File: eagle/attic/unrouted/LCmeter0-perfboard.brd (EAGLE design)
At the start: 51.1 x 49.5 mm, 25 parts, among them IC1 PIC16F876A-X/SP, K2 DS2Y, Q1 20MHz, Q2 BC548, SW1 SPST, SW2 DPDT

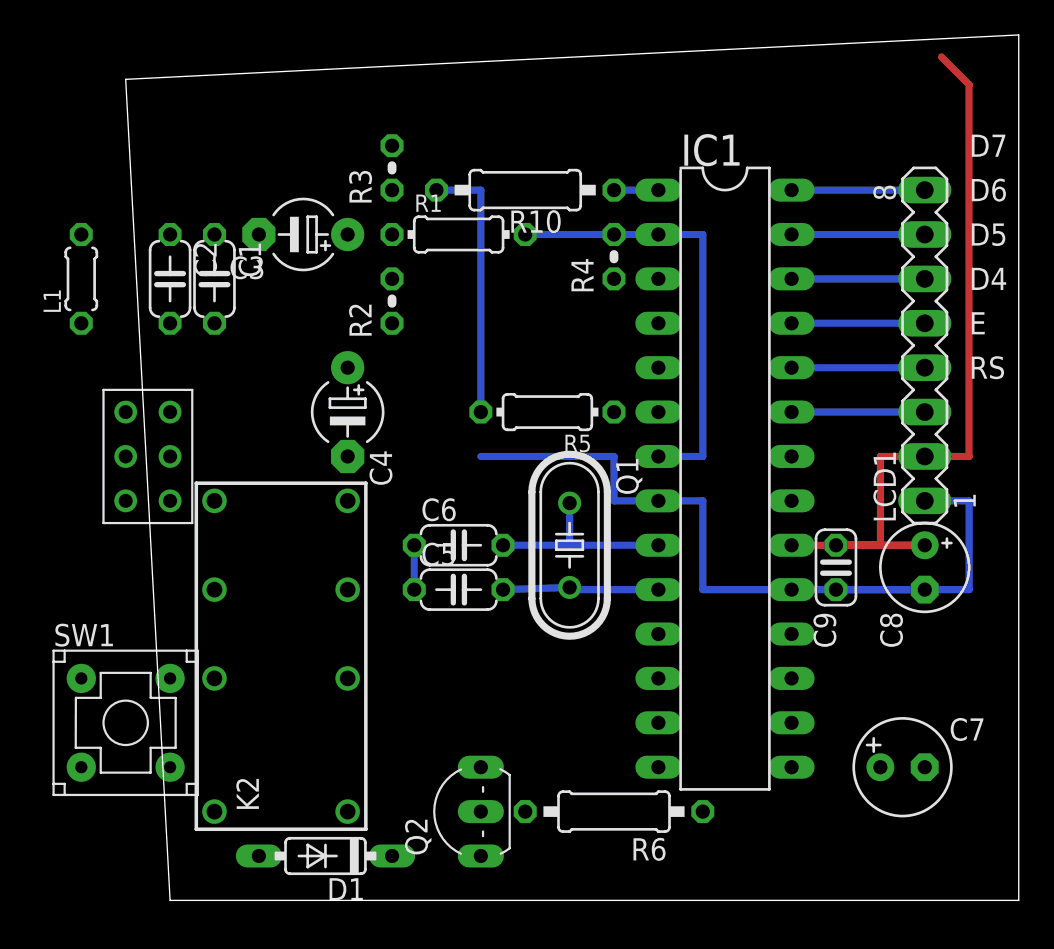
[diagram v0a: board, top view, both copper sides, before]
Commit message: ...
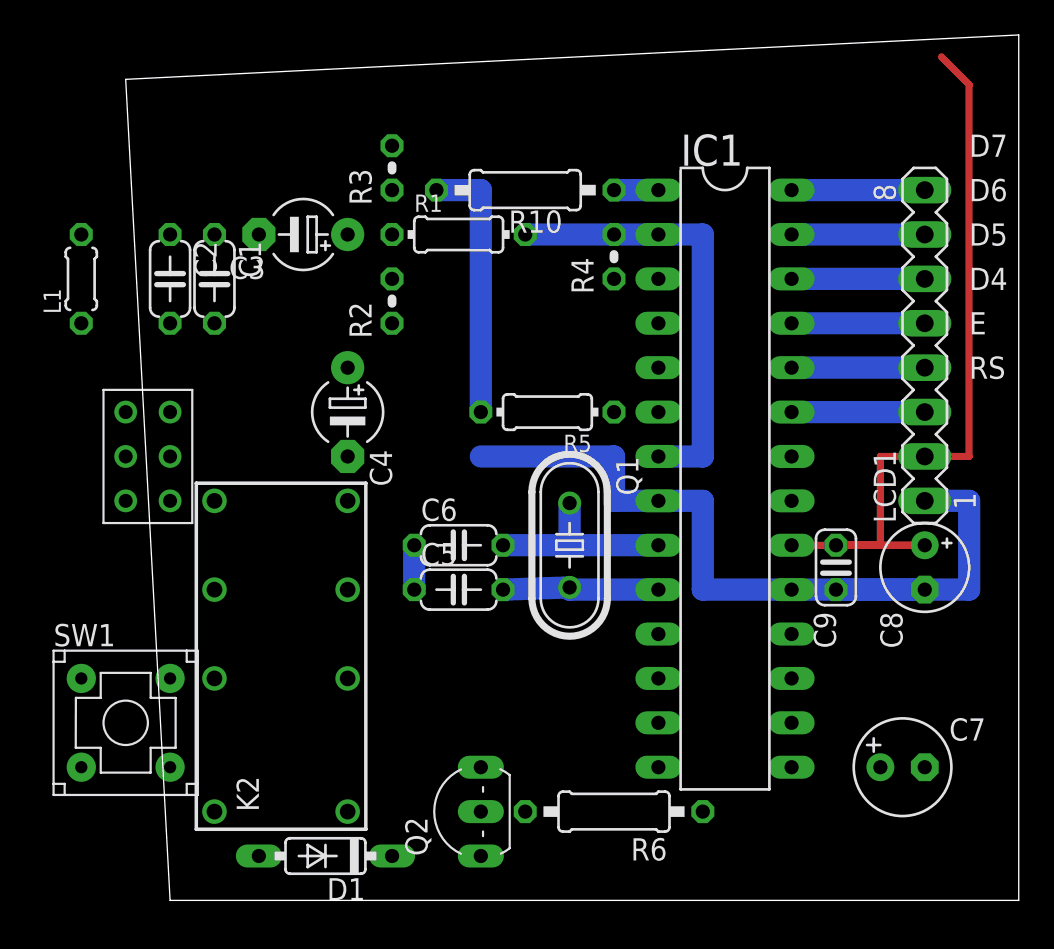
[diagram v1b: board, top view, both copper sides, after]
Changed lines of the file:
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@@
 <contactref element="IC1" pad="2"/>
 <contactref element="IC1" pad="7"/>
-<wire x1="27.94" y1="25.4" x2="30.48" y2="25.4" width="0.4064" layer="16"/>
-<wire x1="30.48" y1="25.4" x2="30.48" y2="38.1" width="0.4064" layer="16"/>
-<wire x1="30.48" y1="38.1" x2="27.94" y2="38.1" width="0.4064" layer="16"/>
-<wire x1="20.32" y1="38.1" x2="25.4" y2="38.1" width="0.4064" layer="16"/>
-<wire x1="25.4" y1="38.1" x2="27.94" y2="38.1" width="0.4064" layer="16"/>
+<wire x1="27.94" y1="25.4" x2="30.48" y2="25.4" width="1.27" layer="16"/>
+<wire x1="30.48" y1="25.4" x2="30.48" y2="38.1" width="1.27" layer="16"/>
+<wire x1="30.48" y1="38.1" x2="27.94" y2="38.1" width="1.27" layer="16"/>
+<wire x1="20.32" y1="38.1" x2="25.4" y2="38.1" width="1.27" layer="16"/>
+<wire x1="25.4" y1="38.1" x2="27.94" y2="38.1" width="1.27" layer="16"/>
 </signal>
 <signal name="A1">
@@
 <contactref element="LCD1" pad="1"/>
 <contactref element="K2" pad="8"/>
-<wire x1="43.18" y1="22.86" x2="45.72" y2="22.86" width="0.4064" layer="16"/>
-<wire x1="45.72" y1="22.86" x2="45.72" y2="17.78" width="0.4064" layer="16"/>
-<wire x1="45.72" y1="17.78" x2="43.18" y2="17.78" width="0.4064" layer="16"/>
-<wire x1="43.18" y1="17.78" x2="38.1" y2="17.78" width="0.4064" layer="16"/>
-<wire x1="35.56" y1="17.78" x2="43.18" y2="17.78" width="0.4064" layer="16"/>
-<wire x1="35.56" y1="17.78" x2="30.48" y2="17.78" width="0.4064" layer="16"/>
-<wire x1="30.48" y1="17.78" x2="30.48" y2="22.86" width="0.4064" layer="16"/>
-<wire x1="30.48" y1="22.86" x2="27.94" y2="22.86" width="0.4064" layer="16"/>
-<wire x1="25.4" y1="25.4" x2="25.4" y2="22.86" width="0.4064" layer="16"/>
-<wire x1="25.4" y1="22.86" x2="27.94" y2="22.86" width="0.4064" layer="16"/>
-<wire x1="13.97" y1="17.78" x2="13.97" y2="20.32" width="0.4064" layer="16"/>
-<wire x1="25.4" y1="25.4" x2="17.78" y2="25.4" width="0.4064" layer="16"/>
+<wire x1="43.18" y1="22.86" x2="45.72" y2="22.86" width="1.27" layer="16"/>
+<wire x1="45.72" y1="22.86" x2="45.72" y2="17.78" width="1.27" layer="16"/>
+<wire x1="45.72" y1="17.78" x2="43.18" y2="17.78" width="1.27" layer="16"/>
+<wire x1="43.18" y1="17.78" x2="38.1" y2="17.78" width="1.27" layer="16"/>
+<wire x1="35.56" y1="17.78" x2="43.18" y2="17.78" width="1.27" layer="16"/>
+<wire x1="35.56" y1="17.78" x2="30.48" y2="17.78" width="1.27" layer="16"/>
+<wire x1="30.48" y1="17.78" x2="30.48" y2="22.86" width="1.27" layer="16"/>
+<wire x1="30.48" y1="22.86" x2="27.94" y2="22.86" width="1.27" layer="16"/>
+<wire x1="25.4" y1="25.4" x2="25.4" y2="22.86" width="1.27" layer="16"/>
+<wire x1="25.4" y1="22.86" x2="27.94" y2="22.86" width="1.27" layer="16"/>
+<wire x1="13.97" y1="17.78" x2="13.97" y2="20.32" width="1.27" layer="16"/>
+<wire x1="25.4" y1="25.4" x2="17.78" y2="25.4" width="1.27" layer="16"/>
 <wire x1="43.18" y1="17.78" x2="43.18" y2="7.62" width="0" layer="19" extent="1-1"/>
 <wire x1="13.97" y1="20.32" x2="17.78" y2="25.4" width="0" layer="19" extent="16-16"/>
@@
 <contactref element="Q1" pad="1"/>
 <contactref element="IC1" pad="9"/>
-<wire x1="27.94" y1="20.32" x2="22.86" y2="20.32" width="0.4064" layer="16"/>
-<wire x1="22.86" y1="20.32" x2="22.86" y2="22.733" width="0.4064" layer="16"/>
-<wire x1="19.05" y1="20.32" x2="22.86" y2="20.32" width="0.4064" layer="16"/>
+<wire x1="27.94" y1="20.32" x2="22.86" y2="20.32" width="1.27" layer="16"/>
+<wire x1="22.86" y1="20.32" x2="22.86" y2="22.733" width="1.27" layer="16"/>
+<wire x1="19.05" y1="20.32" x2="22.86" y2="20.32" width="1.27" layer="16"/>
 </signal>
 <signal name="OSC2">
@@
 <contactref element="Q1" pad="2"/>
 <contactref element="IC1" pad="10"/>
-<wire x1="27.94" y1="17.78" x2="22.86" y2="17.78" width="0.4064" layer="16"/>
-<wire x1="22.86" y1="17.78" x2="22.86" y2="17.907" width="0.4064" layer="16"/>
-<wire x1="22.86" y1="17.907" x2="19.05" y2="17.78" width="0.4064" layer="16"/>
+<wire x1="27.94" y1="17.78" x2="22.86" y2="17.78" width="1.27" layer="16"/>
+<wire x1="22.86" y1="17.78" x2="22.86" y2="17.907" width="1.27" layer="16"/>
+<wire x1="22.86" y1="17.907" x2="19.05" y2="17.78" width="1.27" layer="16"/>
 </signal>
 <signal name="VCC">
@@
 <wire x1="38.1" y1="20.32" x2="43.18" y2="20.32" width="0.4064" layer="1"/>
 <wire x1="43.18" y1="20.32" x2="35.56" y2="20.32" width="0.4064" layer="1"/>
-<wire x1="15.24" y1="40.64" x2="17.78" y2="40.64" width="0.4064" layer="16"/>
-<wire x1="17.78" y1="40.64" x2="17.78" y2="27.94" width="0.4064" layer="16"/>
+<wire x1="15.24" y1="40.64" x2="17.78" y2="40.64" width="1.27" layer="16"/>
+<wire x1="17.78" y1="40.64" x2="17.78" y2="27.94" width="1.27" layer="16"/>
 <wire x1="15.24" y1="40.64" x2="12.7" y2="43.18" width="0" layer="19" extent="1-1"/>
 <wire x1="35.56" y1="20.32" x2="17.78" y2="27.94" width="0" layer="19" extent="1-1"/>
@@
 <contactref element="IC1" pad="25"/>
 <contactref element="LCD1" pad="5"/>
-<wire x1="35.56" y1="33.02" x2="43.18" y2="33.02" width="0.4064" layer="16"/>
+<wire x1="35.56" y1="33.02" x2="43.18" y2="33.02" width="1.27" layer="16"/>
 </signal>
 <signal name="E">
 <contactref element="IC1" pad="24"/>
 <contactref element="LCD1" pad="4"/>
-<wire x1="35.56" y1="30.48" x2="43.18" y2="30.48" width="0.4064" layer="16"/>
+<wire x1="35.56" y1="30.48" x2="43.18" y2="30.48" width="1.27" layer="16"/>
 </signal>
 <signal name="RS">
 <contactref element="IC1" pad="23"/>
 <contactref element="LCD1" pad="3"/>
-<wire x1="35.56" y1="27.94" x2="43.18" y2="27.94" width="0.4064" layer="16"/>
+<wire x1="35.56" y1="27.94" x2="43.18" y2="27.94" width="1.27" layer="16"/>
 </signal>
 <signal name="A4">
@@
 <contactref element="IC1" pad="1"/>
 <wire x1="0" y1="12.7" x2="25.4" y2="40.64" width="0" layer="19" extent="1-1"/>
-<wire x1="27.94" y1="40.64" x2="25.4" y2="40.64" width="0.4064" layer="16"/>
+<wire x1="27.94" y1="40.64" x2="25.4" y2="40.64" width="1.27" layer="16"/>
 </signal>
 <signal name="RC5">
@@
 <contactref element="LCD1" pad="6"/>
 <contactref element="IC1" pad="26"/>
-<wire x1="35.56" y1="35.56" x2="43.18" y2="35.56" width="0.4064" layer="16"/>
+<wire x1="35.56" y1="35.56" x2="43.18" y2="35.56" width="1.27" layer="16"/>
 </signal>
 <signal name="D6">
 <contactref element="LCD1" pad="7"/>
 <contactref element="IC1" pad="27"/>
-<wire x1="35.56" y1="38.1" x2="43.18" y2="38.1" width="0.4064" layer="16"/>
+<wire x1="35.56" y1="38.1" x2="43.18" y2="38.1" width="1.27" layer="16"/>
 </signal>
 <signal name="D7">
 <contactref element="LCD1" pad="8"/>
 <contactref element="IC1" pad="28"/>
-<wire x1="35.56" y1="40.64" x2="43.18" y2="40.64" width="0.4064" layer="16"/>
+<wire x1="35.56" y1="40.64" x2="43.18" y2="40.64" width="1.27" layer="16"/>
 </signal>
 <signal name="C2_CON">
